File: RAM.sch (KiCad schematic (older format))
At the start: 122 parts, among them Q1 2N7002, Q10 2N7002, Q11 2N7002, Q12 2N7002, Q13 2N7002, Q14 2N7002, Q15 2N7002, Q16 2N7002, Q17 2N7002, Q18 2N7002, Q19 2N7002, Q2 2N7002, Q20 2N7002, Q21 2N7002, Q22 2N7002, Q23 2N7002, Q24 2N7002, Q25 2N7002, Q26 2N7002, Q27 2N7002, Q28 2N7002, Q29 2N7002, Q3 2N7002, Q30 2N7002, Q31 2N7002, Q32 2N7002, Q33 2N7002, Q34 2N7002, Q35 2N7002, Q36 2N7002, Q37 2N7002, Q38 2N7002, Q39 2N7002, Q4 2N7002, Q40 2N7002, Q5 2N7002, Q6 2N7002, Q7 2N7002, Q8 2N7002, Q9 2N7002, U2 IS62WV51216BLL

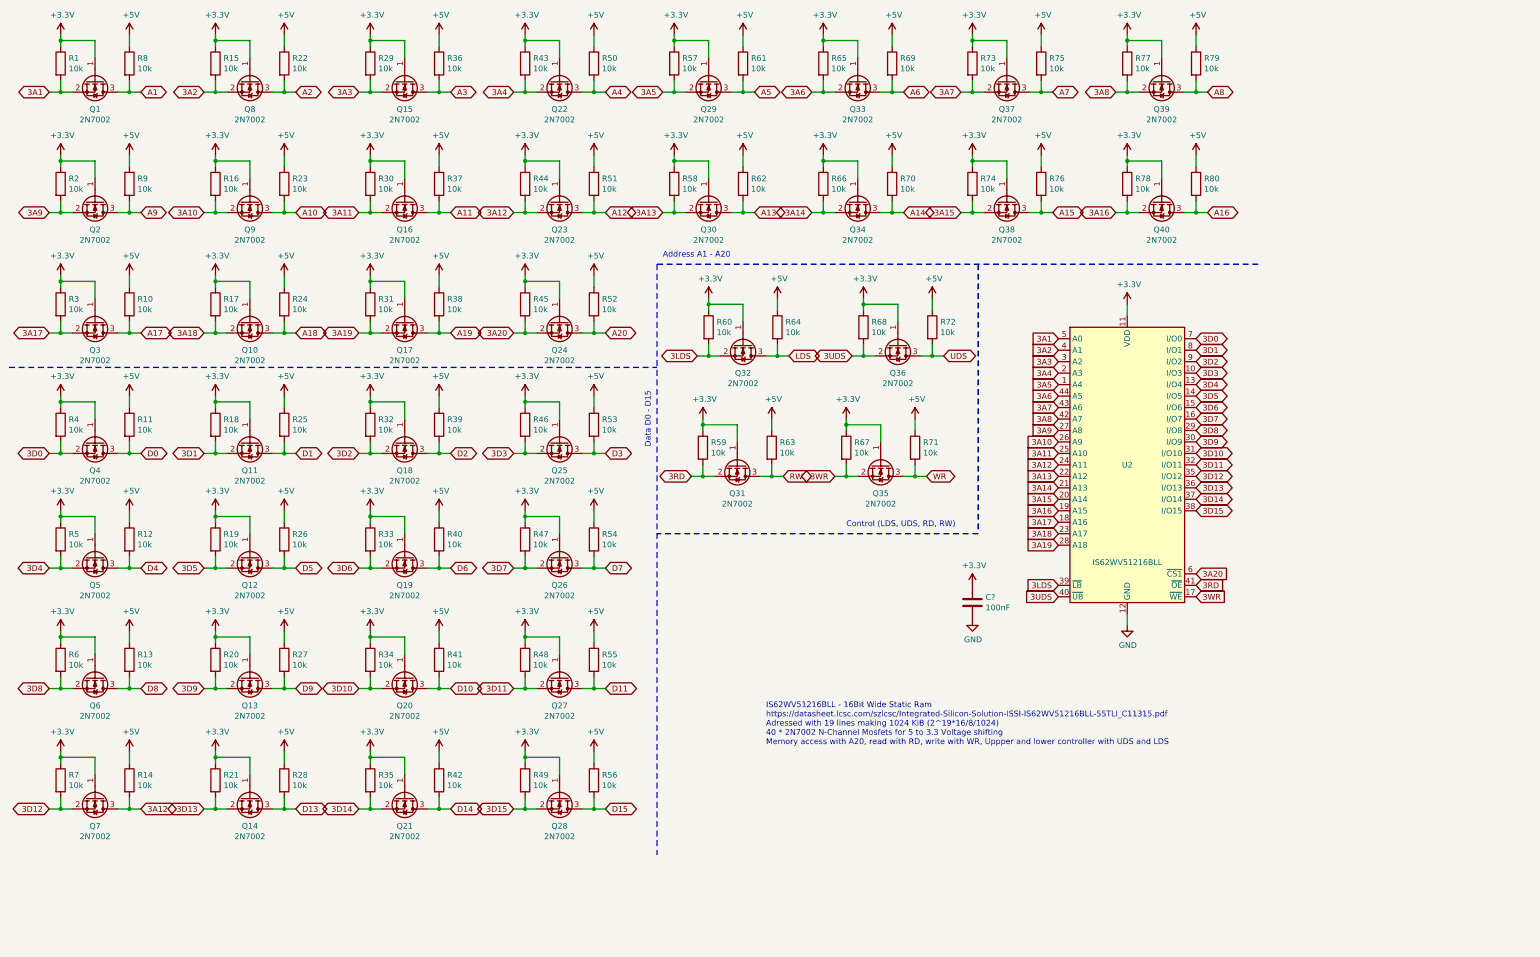
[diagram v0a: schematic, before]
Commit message: updates
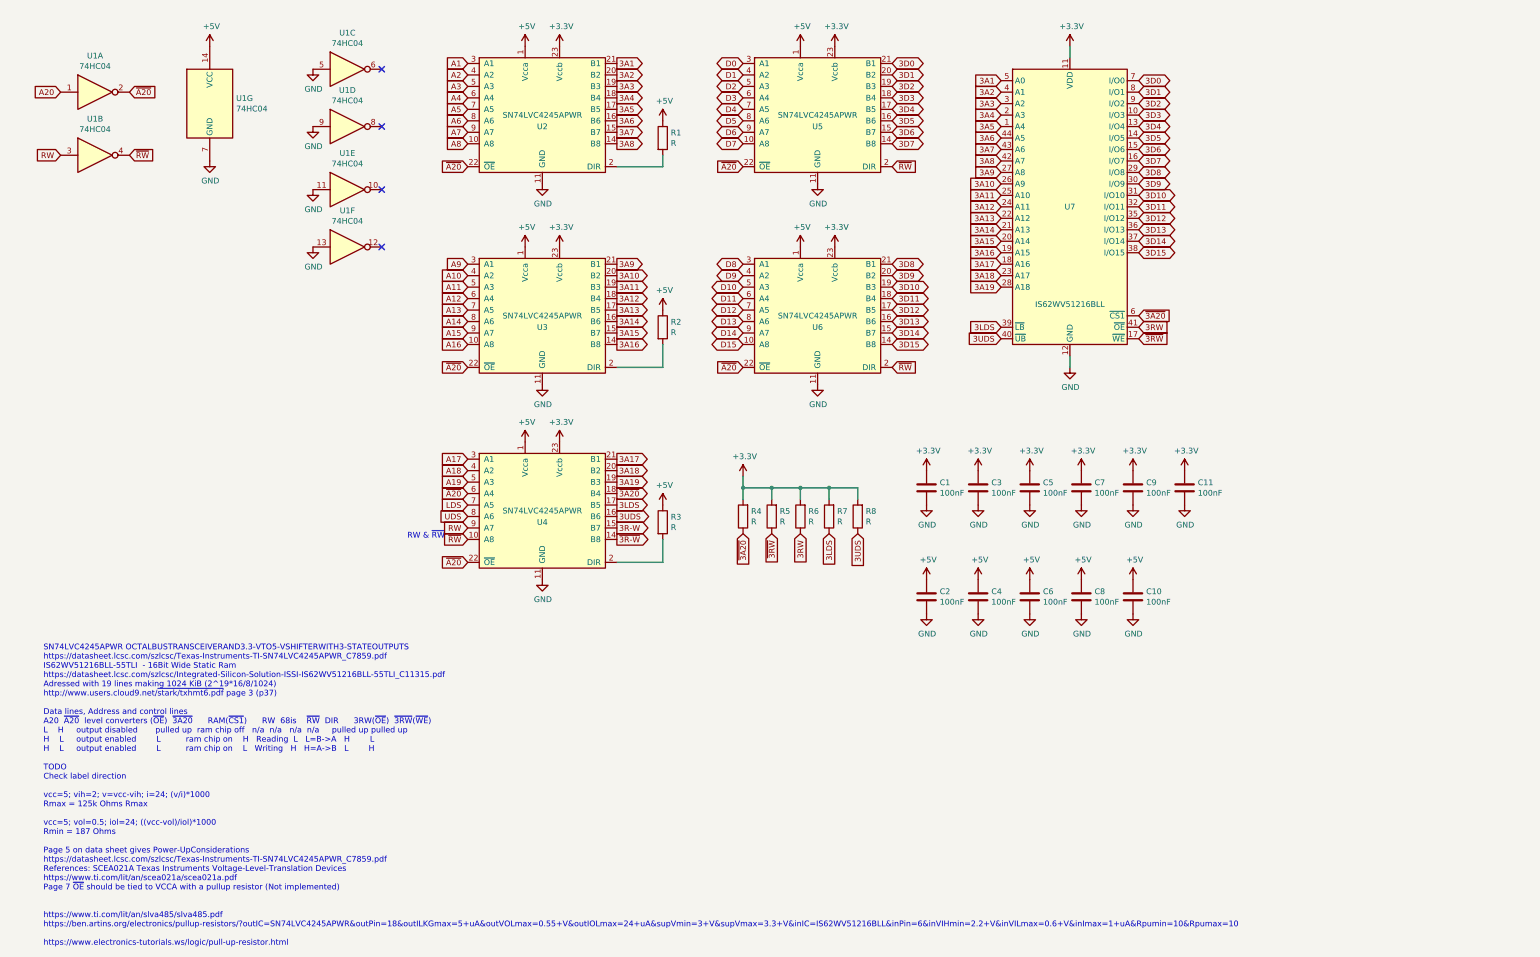
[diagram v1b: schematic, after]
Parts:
- removed Q1, Q10, Q11, Q12, Q13, Q14, Q15, Q16, Q17, Q18, Q19, Q2, Q20, Q21, Q22, Q23, Q24, Q25, Q26, Q27, Q28, Q29, Q3, Q30, Q31, Q32, Q33, Q34, Q35, Q36, Q37, Q38, Q39, Q4, Q40, Q5, Q6, Q7, Q8, Q9: 2N7002, Package_TO_SOT_SMD:SOT-23, symbol Transistor_FET:2N7002
- removed R10, R11, R12, R13, R14, R15, R16, R17, R18, R19, R20, R21, R22, R23, R24, R25, R26, R27, R28, R29, R30, R31, R32, R33, R34, R35, R36, R37, R38, R39, R40, R41, R42, R43, R44, R45, R46, R47, R48, R49, R50, R51, R52, R53, R54, R55, R56, R57, R58, R59, R60, R61, R62, R63, R64, R65, R66, R67, R68, R69, R70, R71, R72, R73, R74, R75, R76, R77, R78, R79, R80, R9: 10k, symbol Device:R
- added C1, C10, C2, C3, C4, C5, C6, C7, C8, C9: 100nF, Capacitor_SMD:C_0603_1608Metric, symbol Device:C
- added U1: 74HC04, Package_SO:SOIC-14_3.9x8.7mm_P1.27mm, symbol 74xx:74HC04
- added U2, U3, U4, U5, U6: SN74LVC4245APWR, Package_SO:TSSOP-24_4.4x7.8mm_P0.65, symbol 68kt:SN74LVC4245APWR
- C11: renamed from C?; footprint (none) -> Capacitor_SMD:C_0603_1608Metric; JLPCB Datasheet (none) -> https://datasheet.lcsc.com/szlcsc/YAGEO-CC0603KRX7R9BB104_C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; JLPCB Part (none) -> CC0603KRX7R9BB104
- R1, R2, R3, R4, R5, R6, R7, R8: value 10k -> R
- renumbered U2 to U7
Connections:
- net +3V3: now also R4.2, R5.2, R6.2, R7.2, R8.2, C1.1, C3.1, C5.1, C7.1, C9.1, U2.23 (Vccb), U2.24 (Vccb), U3.23 (Vccb), U3.24 (Vccb), U4.23 (Vccb), U4.24 (Vccb), U5.23 (Vccb), U5.24 (Vccb), U6.23 (Vccb), U6.24 (Vccb); no longer R1.1, R2.1, R3.1, R4.1, R5.1, R6.1, R7.1
- net +5V: now also R1.1, R2.1, R3.1, C10.1, C2.1, C4.1, C6.1, C8.1, U1.14 (VCC), U2.1 (Vcca), U3.1 (Vcca), U4.1 (Vcca), U5.1 (Vcca), U6.1 (Vcca); no longer R8.1
- net 3A1: now also U2.21 (B1); no longer R1.2
- net 3A10: now also U3.20 (B2)
- net 3A11: now also U3.19 (B3)
- net 3A12: now also U3.18 (B4)
- net 3A13: now also U3.17 (B5)
- net 3A14: now also U3.16 (B6)
- net 3A15: now also U3.15 (B7)
- net 3A16: now also U3.14 (B8)
- net 3A17: now also U4.21 (B1); no longer R3.2
- net 3A18: now also U4.20 (B2)
- net 3A19: now also U4.19 (B3)
- net 3A2: now also U2.20 (B2)
- net 3A3: now also U2.19 (B3)
- net 3A4: now also U2.18 (B4)
- net 3A5: now also U2.17 (B5)
- net 3A6: now also U2.16 (B6)
- net 3A7: now also U2.15 (B7)
- net 3A8: now also U2.14 (B8)
- net 3A9: now also U3.21 (B1); no longer R2.2
- net 3D0: now also U5.21 (B1); no longer R4.2
- net 3D1: now also U5.20 (B2)
- net 3D10: now also U6.19 (B3)
- net 3D11: now also U6.18 (B4)
- net 3D12: now also U6.17 (B5); no longer R7.2
- net 3D13: now also U6.16 (B6)
- net 3D14: now also U6.15 (B7)
- net 3D15: now also U6.14 (B8)
- net 3D2: now also U5.19 (B3)
- net 3D3: now also U5.18 (B4)
- net 3D4: now also U5.17 (B5); no longer R5.2
- net 3D5: now also U5.16 (B6)
- net 3D6: now also U5.15 (B7)
- net 3D7: now also U5.14 (B8)
- net 3D8: now also U6.21 (B1); no longer R6.2
- net 3D9: now also U6.20 (B2)
- net 3LDS: now also R7.1, U4.17 (B5)
- net 3UDS: now also R8.1, U4.16 (B6)
- net A1: now also U2.3 (A1); no longer R8.2
- net A10: now also U3.4 (A2)
- net A11: now also U3.5 (A3)
- net A12: now also U3.6 (A4)
- net A13: now also U3.7 (A5)
- net A14: now also U3.8 (A6)
- net A15: now also U3.9 (A7)
- net A16: now also U3.10 (A8)
- net A17: now also U4.3 (A1)
- net A18: now also U4.4 (A2)
- net A19: now also U4.5 (A3)
- net A2: now also U2.4 (A2)
- net A20: now also U1.1
- net A3: now also U2.5 (A3)
- net A4: now also U2.6 (A4)
- net A5: now also U2.7 (A5)
- net A6: now also U2.8 (A6)
- net A7: now also U2.9 (A7)
- net A8: now also U2.10 (A8)
- net A9: now also U3.3 (A1)
- net D0: now also U5.3 (A1)
- net D1: now also U5.4 (A2)
- net D10: now also U6.5 (A3)
- net D11: now also U6.6 (A4)
- net D13: now also U6.8 (A6)
- net D14: now also U6.9 (A7)
- net D15: now also U6.10 (A8)
- net D2: now also U5.5 (A3)
- net D3: now also U5.6 (A4)
- net D4: now also U5.7 (A5)
- net D5: now also U5.8 (A6)
- net D6: now also U5.9 (A7)
- net D7: now also U5.10 (A8)
- net D8: now also U6.3 (A1)
- net D9: now also U6.4 (A2)
- net GND: now also C1.2, C10.2, C2.2, C3.2, C4.2, C5.2, C6.2, C7.2, C8.2, C9.2, U1.11, U1.13, U1.5, U1.7 (GND), U1.9, U2.11 (GND), U2.12 (GND), U2.13 (GND), U3.11 (GND), U3.12 (GND), U3.13 (GND), U4.11 (GND), U4.12 (GND), U4.13 (GND), U5.11 (GND), U5.12 (GND), U5.13 (GND), U6.11 (GND), U6.12 (GND), U6.13 (GND)
- net LDS: now also U4.7 (A5)
- net RW: now also U1.3, U4.9 (A7)
- net UDS: now also U4.8 (A6)
- net 3A20 renamed ~3A20
- net ~3A20: now also R4.1, U4.18 (B4)
- net 3RD renamed 3RW
- net 3RW: now also R6.1
- net 3WR renamed ~3RW
- net ~3RW: now also R5.1
- new net: R1.2, U2.2 (DIR)
- new net: R2.2, U3.2 (DIR)
- new net: R3.2, U4.2 (DIR)
- new net 3R-W: U4.15 (B7)
- new net D12: U6.7 (A5)
- new net ~3R-W: U4.14 (B8)
- new net ~A20: U1.2, U2.22 (~OE), U3.22 (~OE), U4.22 (~OE), U4.6 (A4), U5.22 (~OE), U6.22 (~OE)
- new net ~RW: U1.4, U4.10 (A8), U5.2 (DIR), U6.2 (DIR)
- no-connect marks 0 -> 4
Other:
- note added: "RW & ~RW~"
- note added: "SN74LVC4245APWR OCTALBUSTRANSCEIVERAND3.3-VTO5-VSHIFTERWITH3-STATEOUTPUTS\nhttps://datasheet.lcsc.com/szlcsc/Texas-Instruments-TI-SN74LVC4245APWR_C7859.pdf\nIS62WV51216BLL-55TLI - 16Bit Wide Static Ram\nhttps://datasheet.lcsc.com/szlcsc/Integrated-Silicon-Solution-ISSI-IS62WV51216BLL-55TLI_C11315.pdf\nAdressed with 19 lines making 1024 KiB (2^19*16/8/1024)\nhttp://www.users.cloud9.net/~stark/txhm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"
- note removed: "Address A1 - A20"
- note removed: "Control (LDS, UDS, RD, RW)"
- note removed: "Data D0 - D15"
- note removed: "IS62WV51216BLL - 16Bit Wide Static Ram\nhttps://datasheet.lcsc.com/szlcsc/Integrated-Silicon-Solution-ISSI-IS62WV51216BLL-55TLI_C11315.pdf\nAdressed with 19 lines making 1024 KiB (2^19*16/8/1024)\n40 * 2N7002 N-Channel Mosfets for 5 to 3.3 Voltage shifting\nMemory access with A20, read with RD, write with WR, Uppper and lower controller with UDS and LDS"
- moved on the sheet: C11, U7

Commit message: updates
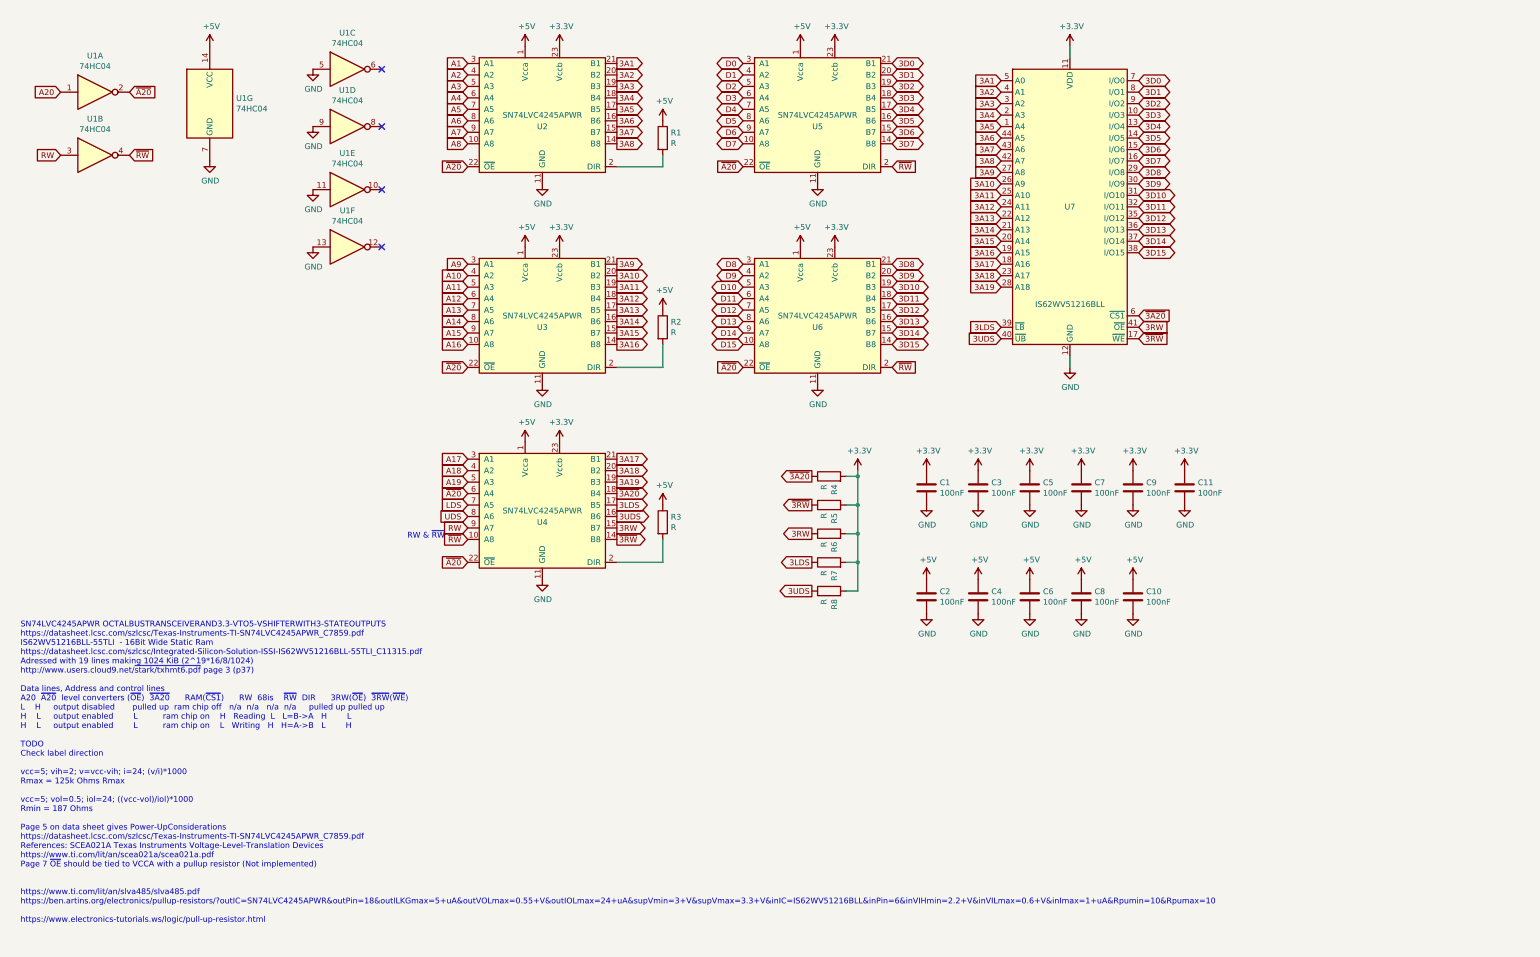
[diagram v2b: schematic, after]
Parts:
- U2, U3, U4, U5, U6: footprint Package_SO:TSSOP-24_4.4x7.8mm_P0.65 -> Package_SO:TSSOP-24_4.4x7.8mm_P0.65mm; JLPCB Datasheet (none) -> https://datasheet.lcsc.com/szlcsc/Texas-Instruments-TI-SN74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; JLPCB Part (none) -> SN74LVC4245APWR
- U7: JLPCB Datasheet (none) -> https://datasheet.lcsc.com/szlcsc/Integrated-Silicon-Soluti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; JLPCB Part (none) -> IS62WV51216BLL-55TLI
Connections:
- net 3R-W is gone; now on net 3RW: U4.15 (B7)
- net ~3R-W is gone; now on net ~3RW: U4.14 (B8)

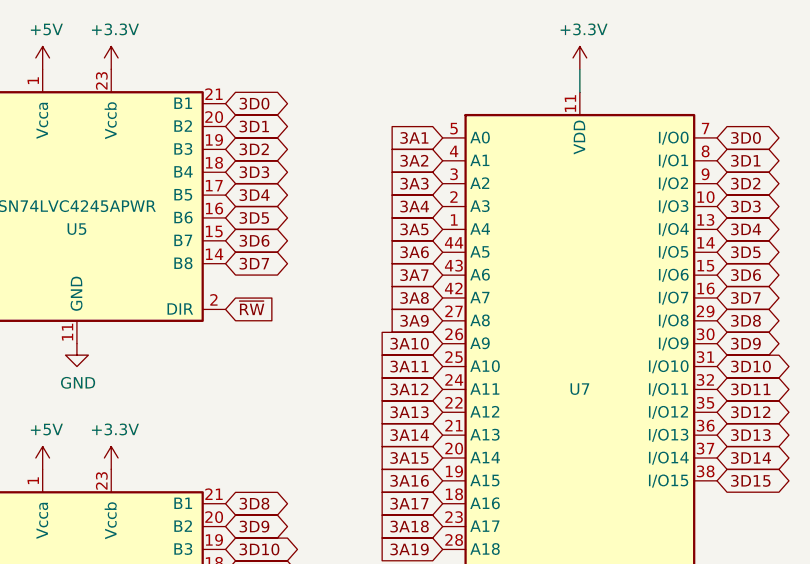
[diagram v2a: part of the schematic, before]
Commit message: update
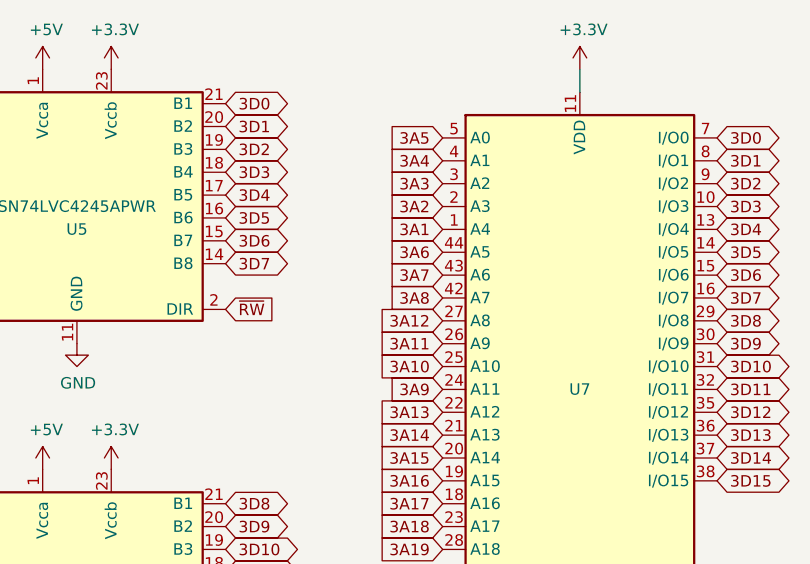
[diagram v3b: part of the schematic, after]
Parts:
- R1, R2, R3, R4, R5, R6, R7, R8: footprint (none) -> Resistor_SMD:R_0603_1608Metric
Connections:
- net 3A1: now also U7.1 (A4); no longer U7.5 (A0)
- net 3A10: now also U7.25 (A10); no longer U7.26 (A9)
- net 3A11: now also U7.26 (A9); no longer U7.25 (A10)
- net 3A12: now also U7.27 (A8); no longer U7.24 (A11)
- net 3A2: now also U7.2 (A3); no longer U7.4 (A1)
- net 3A4: now also U7.4 (A1); no longer U7.2 (A3)
- net 3A5: now also U7.5 (A0); no longer U7.1 (A4)
- net 3A9: now also U7.24 (A11); no longer U7.27 (A8)
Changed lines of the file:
@@
 Text GLabel 9050 2350 0    50   Input ~ 0
 3A13
-Text GLabel 9050 2250 0    50   Input ~ 0
-3A12
-Text GLabel 9050 2150 0    50   Input ~ 0
-3A11
-Text GLabel 9050 2050 0    50   Input ~ 0
-3A10
-Text GLabel 9050 1950 0    50   Input ~ 0
-3A9
 Text GLabel 9050 1850 0    50   Input ~ 0
 3A8
@@
 Text GLabel 9050 1650 0    50   Input ~ 0
 3A6
-Text GLabel 9050 1550 0    50   Input ~ 0
+Text GLabel 9050 1150 0    50   Input ~ 0
 3A5
-Text GLabel 9050 1450 0    50   Input ~ 0
+Text GLabel 9050 1250 0    50   Input ~ 0
 3A4
 Text GLabel 9050 1350 0    50   Input ~ 0
 3A3
-Text GLabel 9050 1250 0    50   Input ~ 0
+Text GLabel 9050 1450 0    50   Input ~ 0
 3A2
 Text GLabel 10250 2650 2    50   BiDi ~ 0
@@
 Text GLabel 10250 1250 2    50   BiDi ~ 0
 3D1
-Text GLabel 9050 1150 0    50   Input ~ 0
+Text GLabel 9050 1550 0    50   Input ~ 0
 3A1
 $Comp
@@
 F 0 "R2" H 6170 3346 50  0000 L CNN
 F 1 "R" H 6170 3255 50  0000 L CNN
-F 2 "" V 6030 3300 50  0001 C CNN
+F 2 "Resistor_SMD:R_0603_1608Metric" V 6030 3300 50  0001 C CNN
 F 3 "~" H 6100 3300 50  0001 C CNN
 	1    6100 3300
@@
 F 0 "R1" H 6170 1696 50  0000 L CNN
 F 1 "R" H 6170 1605 50  0000 L CNN
-F 2 "" V 6030 1650 50  0001 C CNN
+F 2 "Resistor_SMD:R_0603_1608Metric" V 6030 1650 50  0001 C CNN
 F 3 "~" H 6100 1650 50  0001 C CNN
 	1    6100 1650
@@
 F 0 "R3" H 6170 5046 50  0000 L CNN
 F 1 "R" H 6170 4955 50  0000 L CNN
-F 2 "" V 6030 5000 50  0001 C CNN
+F 2 "Resistor_SMD:R_0603_1608Metric" V 6030 5000 50  0001 C CNN
 F 3 "~" H 6100 5000 50  0001 C CNN
 	1    6100 5000
@@
 F 0 "R4" H 7480 4554 50  0000 R CNN
 F 1 "R" H 7480 4645 50  0000 R CNN
-F 2 "" V 7480 4600 50  0001 C CNN
+F 2 "Resistor_SMD:R_0603_1608Metric" V 7480 4600 50  0001 C CNN
 F 3 "~" H 7550 4600 50  0001 C CNN
 	1    7550 4600
@@
 F 0 "R5" H 7480 4804 50  0000 R CNN
 F 1 "R" H 7480 4895 50  0000 R CNN
-F 2 "" V 7480 4850 50  0001 C CNN
+F 2 "Resistor_SMD:R_0603_1608Metric" V 7480 4850 50  0001 C CNN
 F 3 "~" H 7550 4850 50  0001 C CNN
 	1    7550 4850
@@
 F 0 "R6" H 7480 5054 50  0000 R CNN
 F 1 "R" H 7480 5145 50  0000 R CNN
-F 2 "" V 7480 5100 50  0001 C CNN
+F 2 "Resistor_SMD:R_0603_1608Metric" V 7480 5100 50  0001 C CNN
 F 3 "~" H 7550 5100 50  0001 C CNN
 	1    7550 5100
@@
 F 0 "R7" H 7480 5304 50  0000 R CNN
 F 1 "R" H 7480 5395 50  0000 R CNN
-F 2 "" V 7480 5350 50  0001 C CNN
+F 2 "Resistor_SMD:R_0603_1608Metric" V 7480 5350 50  0001 C CNN
 F 3 "~" H 7550 5350 50  0001 C CNN
 	1    7550 5350
@@
 F 0 "R8" H 7480 5554 50  0000 R CNN
 F 1 "R" H 7480 5645 50  0000 R CNN
-F 2 "" V 7480 5600 50  0001 C CNN
+F 2 "Resistor_SMD:R_0603_1608Metric" V 7480 5600 50  0001 C CNN
 F 3 "~" H 7550 5600 50  0001 C CNN
 	1    7550 5600
@@
 Wire Wire Line
 	7800 4600 7800 4550
+Text GLabel 9050 2250 0    50   Input ~ 0
+3A9
+Text GLabel 9050 2150 0    50   Input ~ 0
+3A10
+Text GLabel 9050 2050 0    50   Input ~ 0
+3A11
+Text GLabel 9050 1950 0    50   Input ~ 0
+3A12
 $EndSCHEMATC
